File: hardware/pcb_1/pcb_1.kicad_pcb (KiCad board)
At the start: 2 copper layers, 50 x 50 mm, 5 parts, among them J1 Connector, USB-TYPE-C-16P

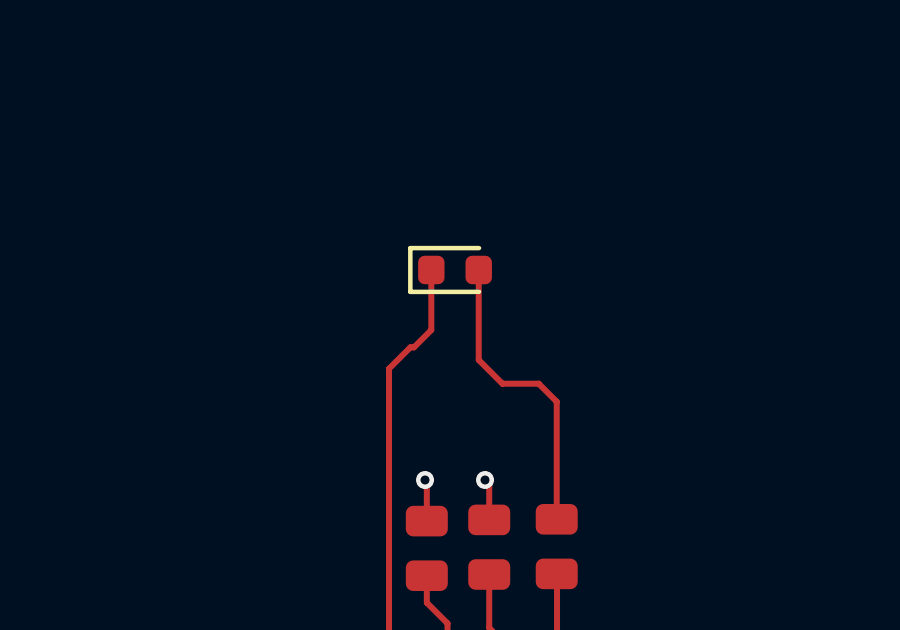
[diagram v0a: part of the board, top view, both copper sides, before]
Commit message: Revert "test change"
This reverts commit c6a32f49c12a29cbde64a1e56dcd0d5c82cf73ba.
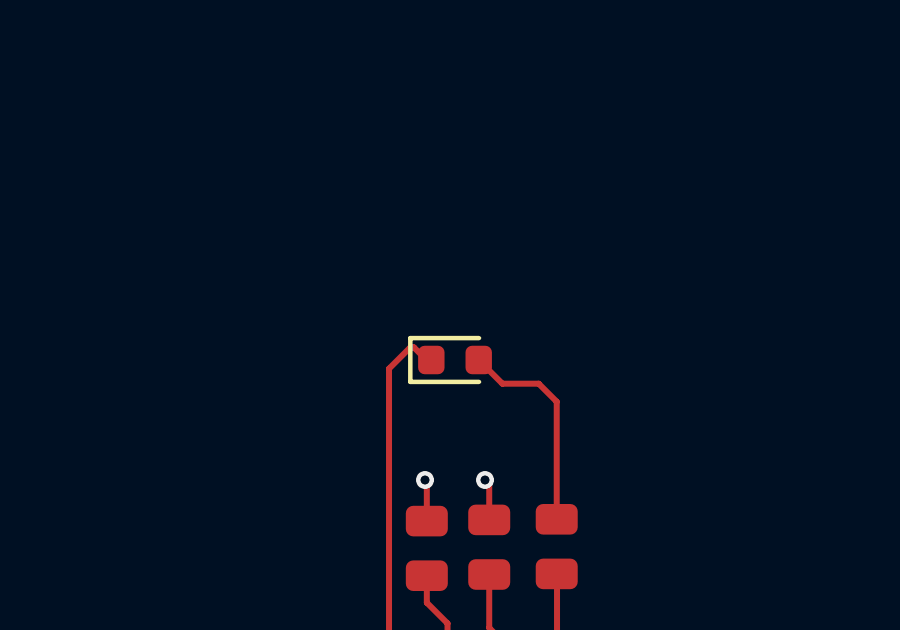
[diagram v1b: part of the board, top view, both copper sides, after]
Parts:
- moved D1 3.00 mm to (116.0, 65.0)
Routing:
- net Net-(D1-Pad2): track 10.1 -> 7.10 mm
- net GND: track 17.9 -> 15.9 mm
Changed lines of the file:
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@@
 	(footprint "PCM_JLCPCB:D_0603"
 		(layer "F.Cu")
-		(at 116 62)
+		(at 116 65)
 		(descr "LED SMD 0603 (1608 Metric), square (rectangular) end terminal, IPC_7351 nominal, (Body size source: http://www.tortai-tech.com/upload/download/2011102023233369053.pdf), generated with kicad-footprint-generator")
 		(tags "LED")
@@
 	)
 	(segment
-		(start 116.79 65)
-		(end 116.79 62)
-		(width 0.2)
-		(layer "F.Cu")
-		(net 1)
-	)
-	(segment
 		(start 119.39 66.39)
 		(end 118.79 65.79)
@@
 	)
 	(segment
+		(start 117.58 65.79)
+		(end 116.79 65)
+		(width 0.2)
+		(layer "F.Cu")
+		(net 1)
+	)
+	(segment
+		(start 118.79 65.79)
+		(end 117.58 65.79)
+		(width 0.2)
+		(layer "F.Cu")
+		(net 1)
+	)
+	(segment
 		(start 119.39 70.31)
 		(end 119.39 66.39)
@@
 	)
 	(segment
-		(start 118.79 65.79)
-		(end 117.58 65.79)
-		(width 0.2)
-		(layer "F.Cu")
-		(net 1)
-	)
-	(segment
-		(start 117.58 65.79)
-		(end 116.79 65)
-		(width 0.2)
-		(layer "F.Cu")
-		(net 1)
-	)
-	(segment
-		(start 114.63 64.58)
-		(end 115.21 64)
+		(start 114.51 64.58)
+		(end 114.63 64.58)
 		(width 0.2)
 		(layer "F.Cu")
@@
 	)
 	(segment
-		(start 114.51 64.58)
-		(end 114.63 64.58)
+		(start 113.8 65.29)
+		(end 114.51 64.58)
+		(width 0.2)
+		(layer "F.Cu")
+		(net 2)
+	)
+	(segment
+		(start 115.05 65)
+		(end 115.21 65)
 		(width 0.2)
 		(layer "F.Cu")
@@
 	)
 	(segment
-		(start 113.8 65.29)
-		(end 114.51 64.58)
-		(width 0.2)
-		(layer "F.Cu")
-		(net 2)
-	)
-	(segment
 		(start 115.06 69.06)
 		(end 115 69)
@@
 	)
 	(segment
-		(start 115.21 64)
-		(end 115.21 62)
-		(width 0.2)
-		(layer "F.Cu")
+		(start 114.63 64.58)
+		(end 115.05 65)
+		(width 0.2)
+		(layer "F.Cu")

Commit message: test change
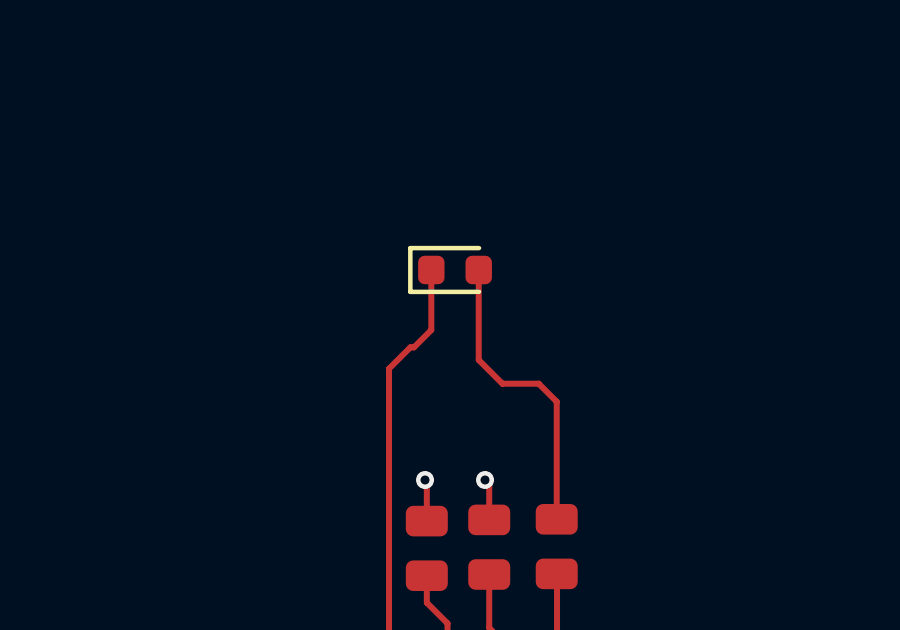
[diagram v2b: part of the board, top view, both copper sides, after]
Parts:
- moved D1 3.00 mm to (116.0, 62.0)
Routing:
- net Net-(D1-Pad2): track 7.10 -> 10.1 mm
- net GND: track 15.9 -> 17.9 mm
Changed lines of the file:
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@@
 	(footprint "PCM_JLCPCB:D_0603"
 		(layer "F.Cu")
-		(at 116 65)
+		(at 116 62)
 		(descr "LED SMD 0603 (1608 Metric), square (rectangular) end terminal, IPC_7351 nominal, (Body size source: http://www.tortai-tech.com/upload/download/2011102023233369053.pdf), generated with kicad-footprint-generator")
 		(tags "LED")
@@
 	)
 	(segment
+		(start 116.79 65)
+		(end 116.79 62)
+		(width 0.2)
+		(layer "F.Cu")
+		(net 1)
+	)
+	(segment
 		(start 119.39 66.39)
 		(end 118.79 65.79)
@@
 	)
 	(segment
+		(start 119.39 70.31)
+		(end 119.39 66.39)
+		(width 0.2)
+		(layer "F.Cu")
+		(net 1)
+	)
+	(segment
+		(start 118.79 65.79)
+		(end 117.58 65.79)
+		(width 0.2)
+		(layer "F.Cu")
+		(net 1)
+	)
+	(segment
 		(start 117.58 65.79)
 		(end 116.79 65)
@@
 	)
 	(segment
-		(start 118.79 65.79)
-		(end 117.58 65.79)
-		(width 0.2)
-		(layer "F.Cu")
-		(net 1)
-	)
-	(segment
-		(start 119.39 70.31)
-		(end 119.39 66.39)
-		(width 0.2)
-		(layer "F.Cu")
-		(net 1)
+		(start 114.63 64.58)
+		(end 115.21 64)
+		(width 0.2)
+		(layer "F.Cu")
+		(net 2)
+	)
+	(segment
+		(start 117.14 70.33)
+		(end 117.14 69.14)
+		(width 0.2)
+		(layer "F.Cu")
+		(net 2)
+	)
+	(segment
+		(start 115.06 70.37)
+		(end 115.06 69.06)
+		(width 0.2)
+		(layer "F.Cu")
+		(net 2)
 	)
 	(segment
@@
 	)
 	(segment
-		(start 117.14 70.33)
-		(end 117.14 69.14)
-		(width 0.2)
-		(layer "F.Cu")
-		(net 2)
-	)
-	(segment
-		(start 115.06 70.37)
-		(end 115.06 69.06)
+		(start 113.8 76.5)
+		(end 113.8 65.29)
 		(width 0.2)
 		(layer "F.Cu")
@@
 	)
 	(segment
-		(start 115.05 65)
-		(end 115.21 65)
-		(width 0.2)
-		(layer "F.Cu")
-		(net 2)
-	)
-	(segment
-		(start 113.8 76.5)
-		(end 113.8 65.29)
-		(width 0.2)
-		(layer "F.Cu")
-		(net 2)
-	)
-	(segment
 		(start 115.06 69.06)
 		(end 115 69)
@@
 	)
 	(segment
-		(start 114.63 64.58)
-		(end 115.05 65)
-		(width 0.2)
-		(layer "F.Cu")
+		(start 115.21 64)
+		(end 115.21 62)
+		(width 0.2)
+		(layer "F.Cu")

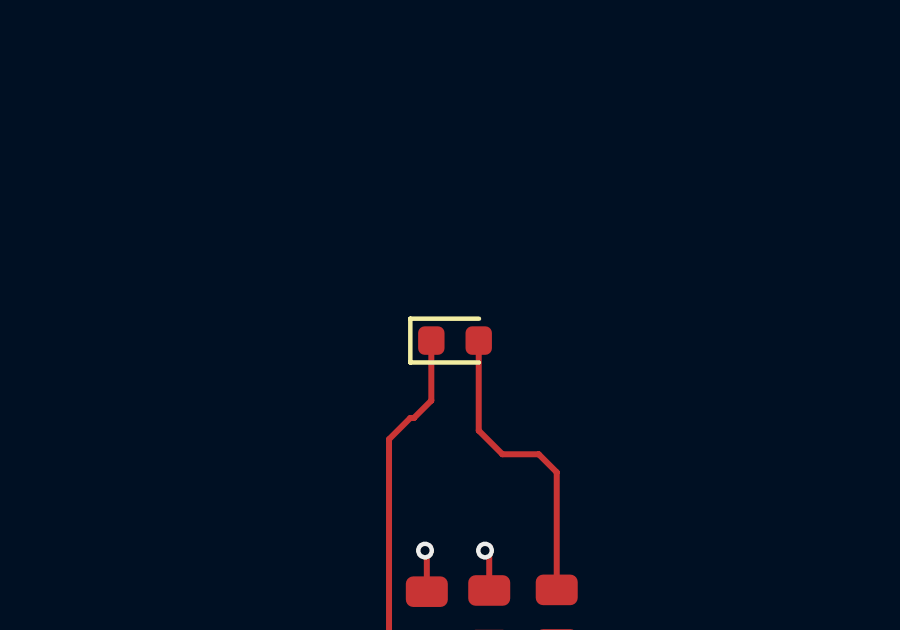
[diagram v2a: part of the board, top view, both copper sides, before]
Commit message: test/workflow-validation
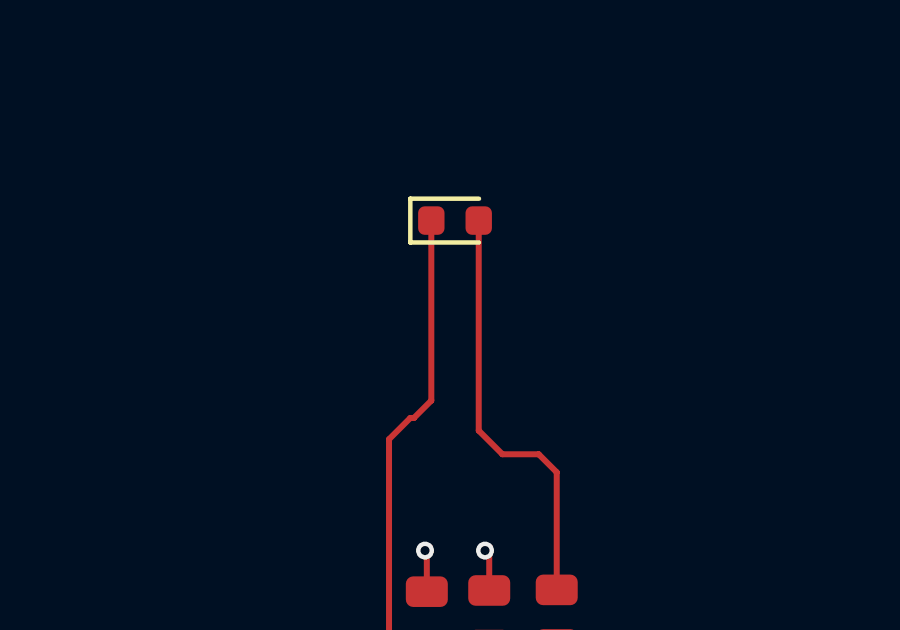
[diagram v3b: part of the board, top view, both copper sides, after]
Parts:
- moved D1 4.00 mm to (116.0, 58.0)
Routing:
- net Net-(D1-Pad2): track 10.1 -> 14.1 mm
- net GND: track 17.9 -> 21.9 mm
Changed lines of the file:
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@@
 	(footprint "PCM_JLCPCB:D_0603"
 		(layer "F.Cu")
-		(at 116 62)
+		(at 116 58)
 		(descr "LED SMD 0603 (1608 Metric), square (rectangular) end terminal, IPC_7351 nominal, (Body size source: http://www.tortai-tech.com/upload/download/2011102023233369053.pdf), generated with kicad-footprint-generator")
 		(tags "LED")
@@
 	)
 	(segment
-		(start 116.79 65)
-		(end 116.79 62)
+		(start 119.39 70.31)
+		(end 119.39 66.39)
+		(width 0.2)
+		(layer "F.Cu")
+		(net 1)
+	)
+	(segment
+		(start 117.58 65.79)
+		(end 116.79 65)
+		(width 0.2)
+		(layer "F.Cu")
+		(net 1)
+	)
+	(segment
+		(start 118.79 65.79)
+		(end 117.58 65.79)
 		(width 0.2)
 		(layer "F.Cu")
@@
 	)
 	(segment
-		(start 119.39 70.31)
-		(end 119.39 66.39)
+		(start 116.79 65)
+		(end 116.79 58)
 		(width 0.2)
 		(layer "F.Cu")
@@
 	)
 	(segment
-		(start 118.79 65.79)
-		(end 117.58 65.79)
-		(width 0.2)
-		(layer "F.Cu")
-		(net 1)
-	)
-	(segment
-		(start 117.58 65.79)
-		(end 116.79 65)
-		(width 0.2)
-		(layer "F.Cu")
-		(net 1)
+		(start 117.14 70.33)
+		(end 117.14 69.14)
+		(width 0.2)
+		(layer "F.Cu")
+		(net 2)
+	)
+	(segment
+		(start 114.51 64.58)
+		(end 114.63 64.58)
+		(width 0.2)
+		(layer "F.Cu")
+		(net 2)
+	)
+	(segment
+		(start 115.06 70.37)
+		(end 115.06 69.06)
+		(width 0.2)
+		(layer "F.Cu")
+		(net 2)
+	)
+	(segment
+		(start 113.8 65.29)
+		(end 114.51 64.58)
+		(width 0.2)
+		(layer "F.Cu")
+		(net 2)
+	)
+	(segment
+		(start 113.8 76.5)
+		(end 113.8 65.29)
+		(width 0.2)
+		(layer "F.Cu")
+		(net 2)
 	)
 	(segment
@@
 	)
 	(segment
-		(start 117.14 70.33)
-		(end 117.14 69.14)
-		(width 0.2)
-		(layer "F.Cu")
-		(net 2)
-	)
-	(segment
-		(start 115.06 70.37)
-		(end 115.06 69.06)
-		(width 0.2)
-		(layer "F.Cu")
-		(net 2)
-	)
-	(segment
-		(start 114.51 64.58)
-		(end 114.63 64.58)
-		(width 0.2)
-		(layer "F.Cu")
-		(net 2)
-	)
-	(segment
-		(start 113.8 76.5)
-		(end 113.8 65.29)
-		(width 0.2)
-		(layer "F.Cu")
-		(net 2)
-	)
-	(segment
-		(start 113.8 65.29)
-		(end 114.51 64.58)
+		(start 115.21 64)
+		(end 115.21 58)
 		(width 0.2)
 		(layer "F.Cu")
@@
 		(width 0.2)
 		(layer "F.Cu")
-		(net 2)
-	)
-	(segment
-		(start 115.21 64)
-		(end 115.21 62)
-		(width 0.2)
-		(layer "F.Cu")

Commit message: Revert "test/workflow-validation"
This reverts commit f41bfac697a76066e7a57eaa081d6dce11ab9e38.
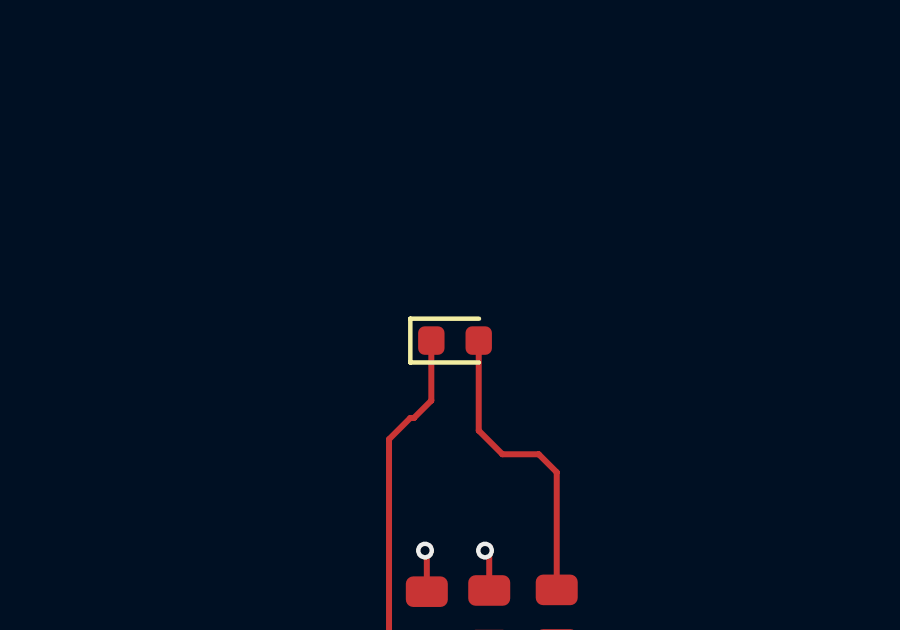
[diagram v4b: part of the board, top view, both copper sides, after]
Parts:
- moved D1 4.00 mm to (116.0, 62.0)
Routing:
- net Net-(D1-Pad2): track 14.1 -> 10.1 mm
- net GND: track 21.9 -> 17.9 mm
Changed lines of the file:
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@@
 	(footprint "PCM_JLCPCB:D_0603"
 		(layer "F.Cu")
-		(at 116 58)
+		(at 116 62)
 		(descr "LED SMD 0603 (1608 Metric), square (rectangular) end terminal, IPC_7351 nominal, (Body size source: http://www.tortai-tech.com/upload/download/2011102023233369053.pdf), generated with kicad-footprint-generator")
 		(tags "LED")
@@
 	)
 	(segment
+		(start 116.79 65)
+		(end 116.79 62)
+		(width 0.2)
+		(layer "F.Cu")
+		(net 1)
+	)
+	(segment
+		(start 119.39 66.39)
+		(end 118.79 65.79)
+		(width 0.2)
+		(layer "F.Cu")
+		(net 1)
+	)
+	(segment
 		(start 119.39 70.31)
 		(end 119.39 66.39)
@@
 	)
 	(segment
+		(start 118.79 65.79)
+		(end 117.58 65.79)
+		(width 0.2)
+		(layer "F.Cu")
+		(net 1)
+	)
+	(segment
 		(start 117.58 65.79)
 		(end 116.79 65)
@@
 	)
 	(segment
-		(start 118.79 65.79)
-		(end 117.58 65.79)
-		(width 0.2)
-		(layer "F.Cu")
-		(net 1)
-	)
-	(segment
-		(start 119.39 66.39)
-		(end 118.79 65.79)
-		(width 0.2)
-		(layer "F.Cu")
-		(net 1)
-	)
-	(segment
-		(start 116.79 65)
-		(end 116.79 58)
-		(width 0.2)
-		(layer "F.Cu")
-		(net 1)
+		(start 114.63 64.58)
+		(end 115.21 64)
+		(width 0.2)
+		(layer "F.Cu")
+		(net 2)
 	)
 	(segment
@@
 	)
 	(segment
+		(start 115.06 70.37)
+		(end 115.06 69.06)
+		(width 0.2)
+		(layer "F.Cu")
+		(net 2)
+	)
+	(segment
 		(start 114.51 64.58)
 		(end 114.63 64.58)
@@
 	)
 	(segment
-		(start 115.06 70.37)
-		(end 115.06 69.06)
+		(start 113.8 76.5)
+		(end 113.8 65.29)
 		(width 0.2)
 		(layer "F.Cu")
@@
 	)
 	(segment
-		(start 113.8 76.5)
-		(end 113.8 65.29)
-		(width 0.2)
-		(layer "F.Cu")
-		(net 2)
-	)
-	(segment
-		(start 114.63 64.58)
-		(end 115.21 64)
-		(width 0.2)
-		(layer "F.Cu")
-		(net 2)
-	)
-	(segment
-		(start 115.21 64)
-		(end 115.21 58)
-		(width 0.2)
-		(layer "F.Cu")
-		(net 2)
-	)
-	(segment
 		(start 115.06 69.06)
 		(end 115 69)
 		(width 0.2)
 		(layer "F.Cu")
+		(net 2)
+	)
+	(segment
+		(start 115.21 64)
+		(end 115.21 62)
+		(width 0.2)
+		(layer "F.Cu")
